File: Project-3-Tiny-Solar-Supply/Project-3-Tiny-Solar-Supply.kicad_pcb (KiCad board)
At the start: 2 copper layers, 40.8 x 19 mm, 16 parts, among them J1 Conn_01x02_Pin, J2 Conn_01x02_Pin, J3 Conn_01x02_Pin, J4 Conn_01x02_Pin, Q1 2N7002, U1 AP3015AKTR-G1

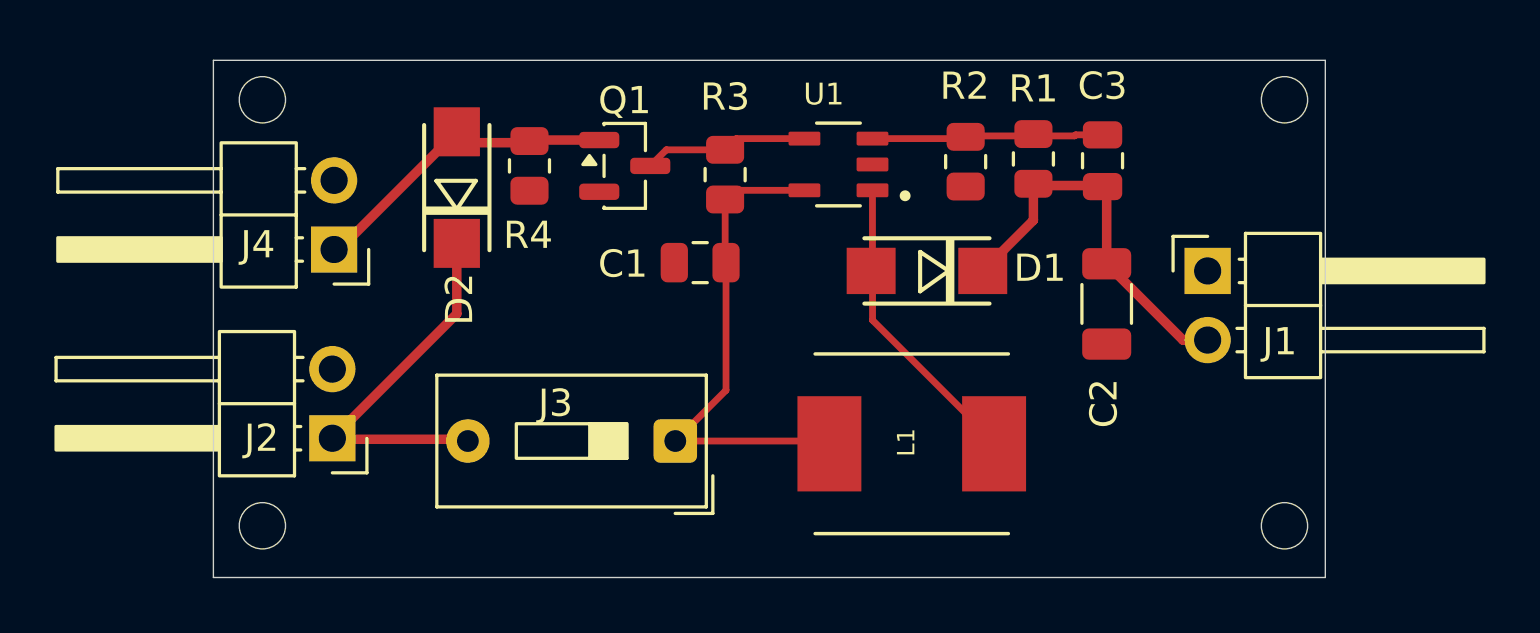
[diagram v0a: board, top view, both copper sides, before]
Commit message: fine re-arrange and wiring, clean up
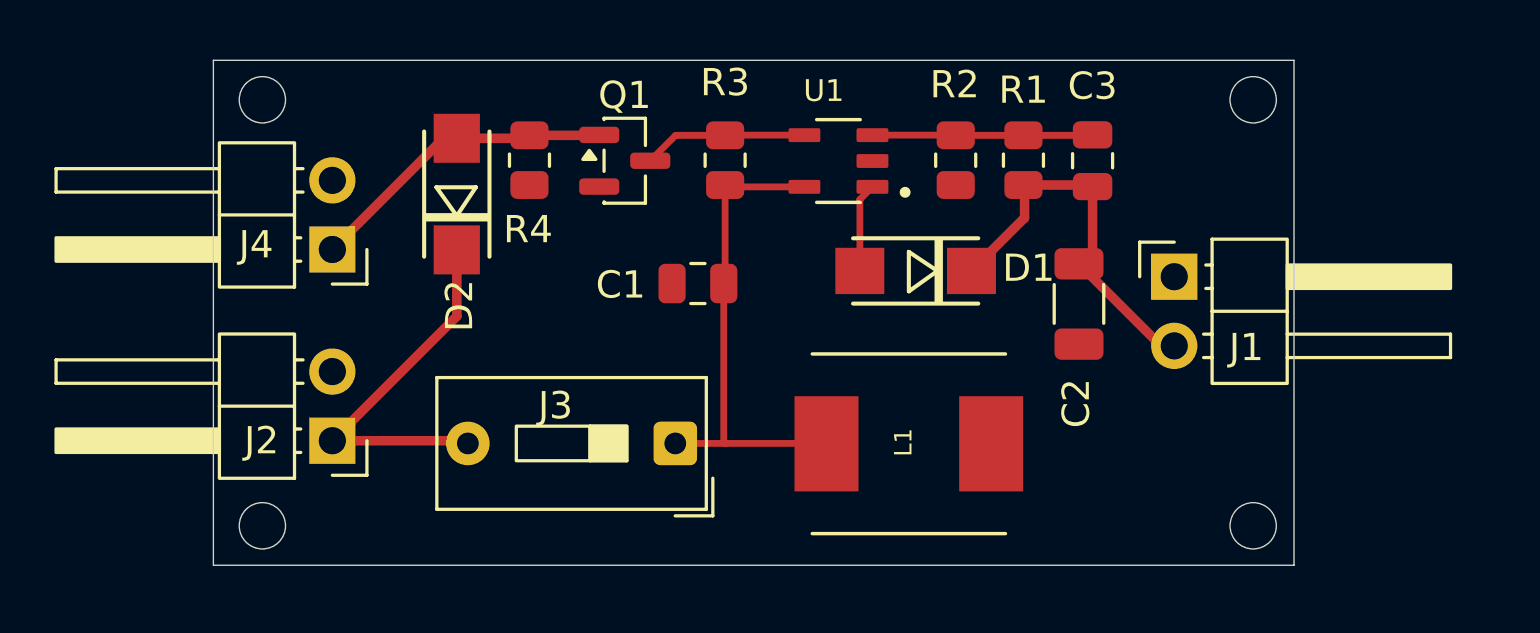
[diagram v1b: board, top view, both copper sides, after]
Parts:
- moved J1 1.25 mm to (73.5, 91.5)
- moved C2 1.02 mm to (70.0, 92.5)
- moved C1 0.77 mm to (56.0, 91.8)
- moved R3 0.53 mm to (57.0, 87.2)
- moved D1 0.41 mm to (64.0, 91.3)
- moved R2 0.37 mm to (65.5, 87.2)
- moved R1 0.37 mm to (68.0, 87.2)
- moved C3 0.37 mm to (70.5, 87.2)
- moved D2 0.24 mm to (47.1, 88.5)
- moved R4 0.21 mm to (49.8, 87.2)
- moved Q1 0.19 mm to (53.3, 87.2)
- moved U1 0.13 mm to (61.2, 87.2)
- moved L1 0.11 mm to (63.8, 97.6)
- moved J2 0.09 mm to (42.6, 97.5)
- moved J3 0.09 mm to (55.2, 97.6)
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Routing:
- net Net-(D1-A): track 11.5 -> 3.28 mm
- net /OUT_P: track 14.8 -> 14.3 mm
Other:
- board size 40.8 x 19 mm -> 39.7 x 18.5 mm
